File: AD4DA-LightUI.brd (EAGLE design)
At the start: 106 x 100 mm, 10 parts

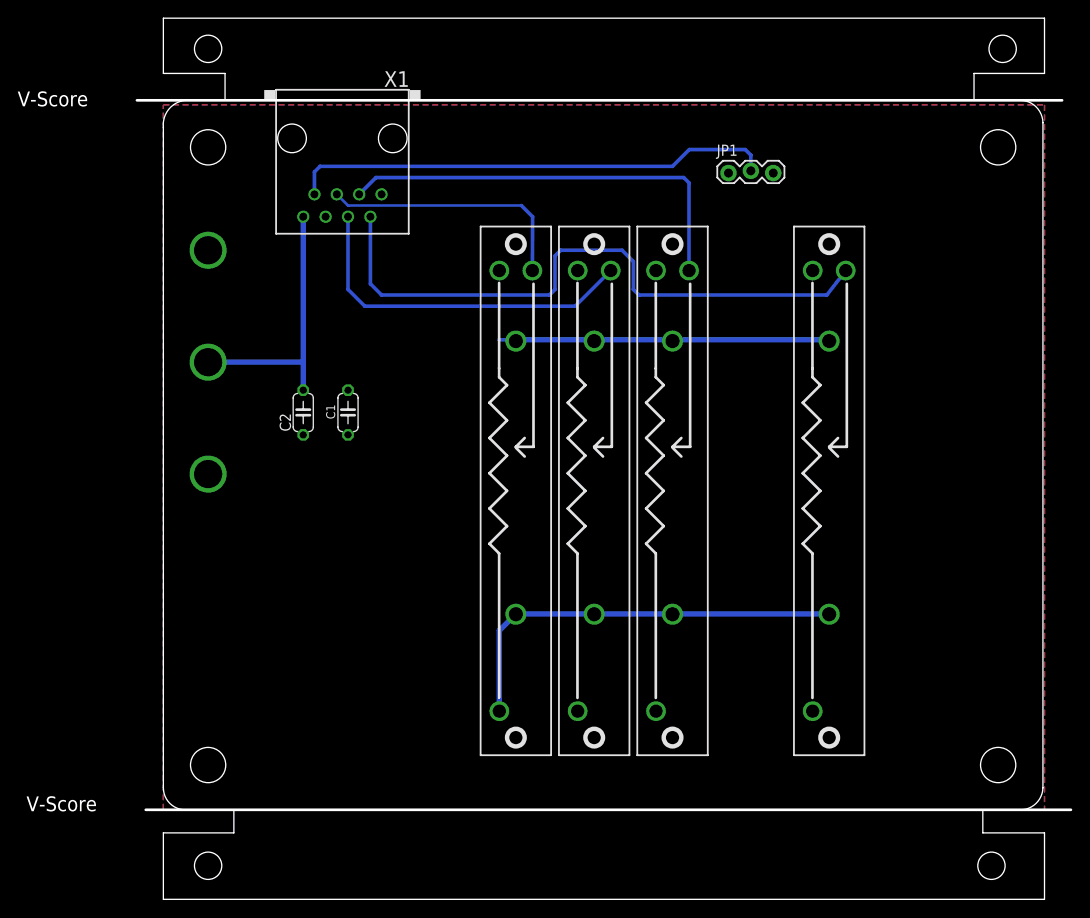
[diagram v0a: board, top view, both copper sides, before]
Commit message: 2.2
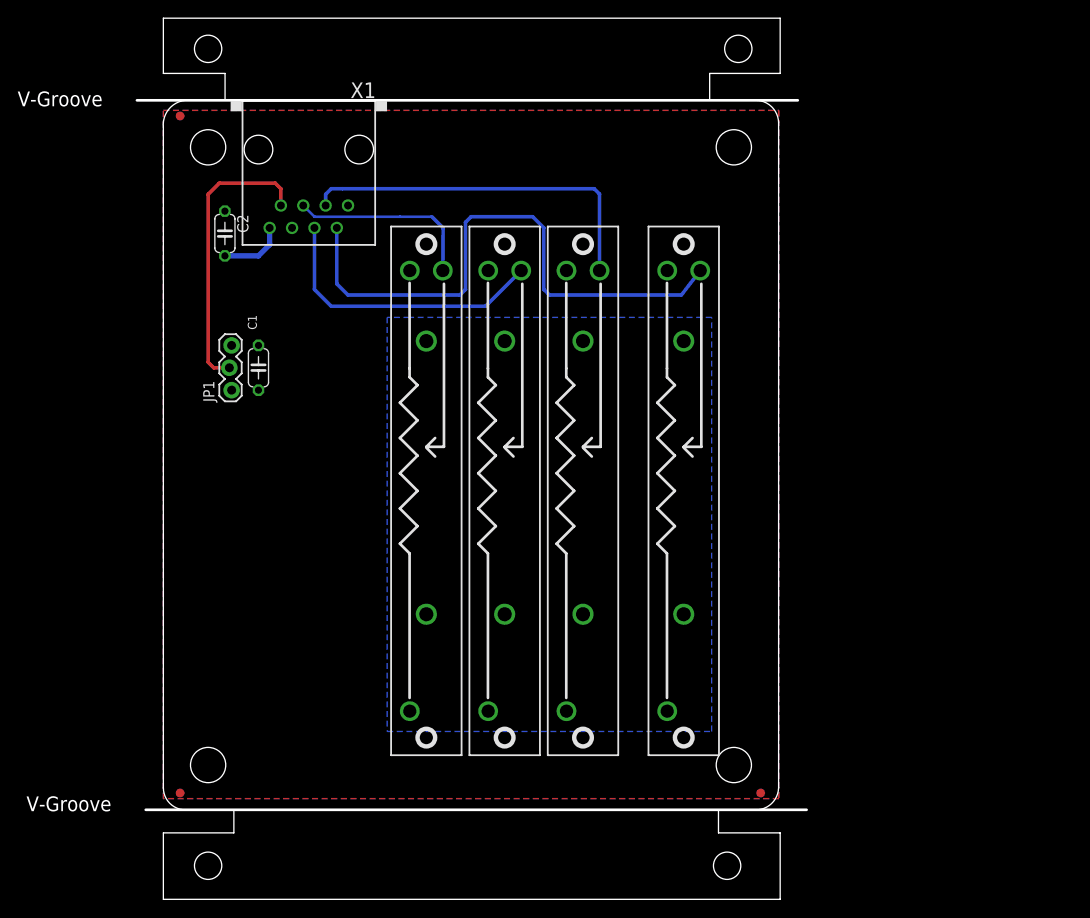
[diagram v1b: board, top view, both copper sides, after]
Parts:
- removed U$1, U$2, U$3, U$7: R-SLIDE-POT-45MM, SPCoast:SLIDER-45MM
- added RS1, RS2, RS3, RS4: 10K OHM "B" TAPER, SPCoast:SLIDER-45MM
- BOARD1: value BOARD80X100 -> 10x7cm; device SPCoast:BOARD-DINRAIL-3.17INX10CM -> SPCoast:BOARD-DINRAIL-3.17INX7CM
- JP1: value JUMPER-3PTH-LOCK -> 1x3
- X1: value (none) -> RJ45/8
- moved LOGO1 69.9 mm to (5.08, 15.2)
- moved JP1 61.7 mm to (7.62, 57.8), turned to 90 degrees
- moved C2 22.2 mm to (6.99, 75.6), turned to 270 degrees
- moved C1 11.4 mm to (10.8, 60.3)
- moved X1 4.02 mm to (16.5, 85.1)
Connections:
- net 5V: now also RS1.E, RS2.E, RS3.E, RS4.E; no longer U$1.E, U$2.E, U$3.E, U$7.E
- net AD0: now also RS4.S; no longer U$7.S
- net AD1: now also RS3.S; no longer U$3.S
- net AD2: now also RS2.S; no longer U$2.S
- net AD3: now also RS1.S; no longer U$1.S
- net AGND: now also RS1.A, RS1.AGND@0, RS1.AGND@1, RS2.A, RS2.AGND@0, RS2.AGND@1, RS3.A, RS3.AGND@0, RS3.AGND@1, RS4.A, RS4.AGND@0, RS4.AGND@1; no longer U$1.A, U$2.A, U$3.A, U$7.A
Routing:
- net AGND: track 84.8 -> 0.00 mm, vias 1 -> 0
- net GND: track 30.5 -> 7.51 mm, vias 1 -> 0
- net DA0: track 55.2 -> 32.7 mm
- net AD2: track 40.5 -> 32.9 mm
- net AD3: track 29.4 -> 21.8 mm
- net AD1: track 48.4 -> 41.6 mm
- net AD0: track 71.8 -> 65.4 mm
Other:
- board size 106 x 100 mm -> 76 x 100 mm
- board text added: "2018-07"
- board text added: "Shrunk board size"
- board text added: "W"
- board text added: "v1.0D"
- board text added: "v2.2"
- board text removed: "2014-12 C"
- board text removed: "Silk Screen mixed AGND and +5V labels"
- board text removed: "White"
- board text removed: "v2.1"
